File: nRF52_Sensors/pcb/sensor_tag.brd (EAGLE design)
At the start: 36.5 x 26.7 mm, 5 parts

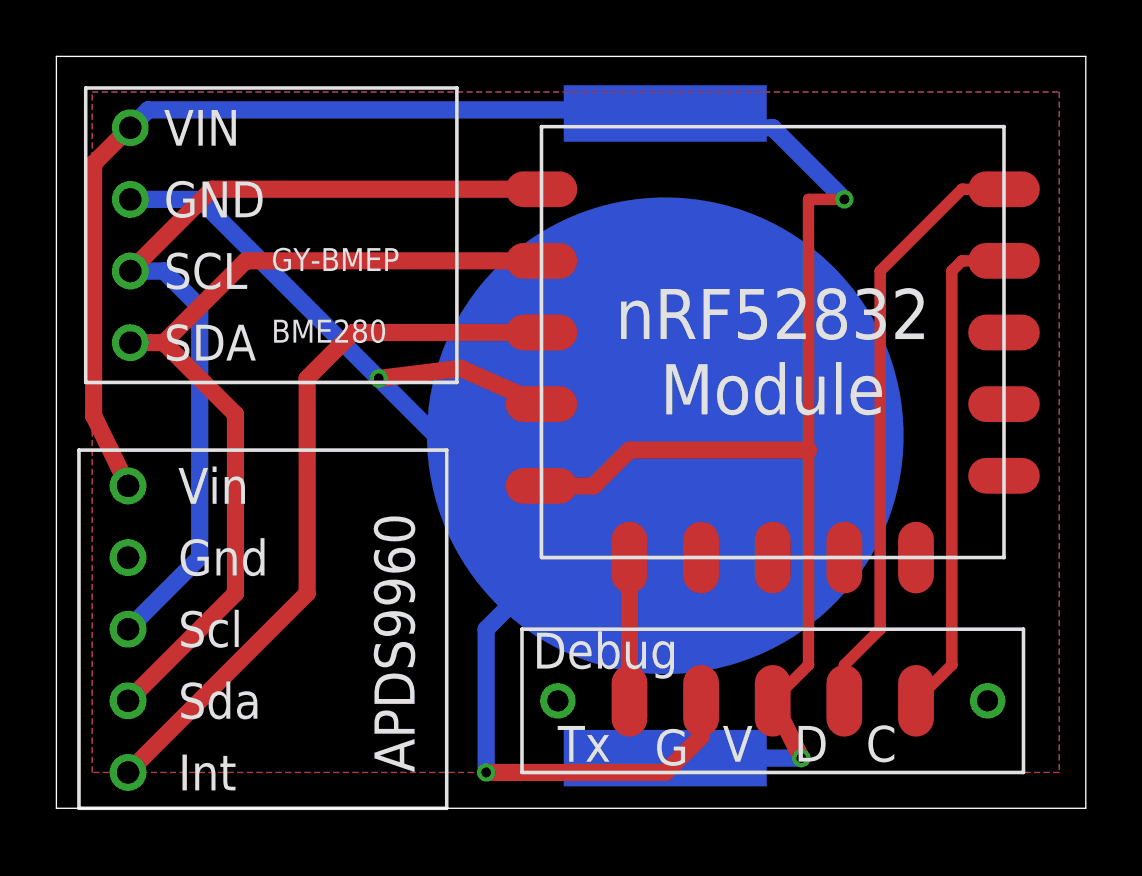
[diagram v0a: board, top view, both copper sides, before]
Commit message: nRF52 tests ongoing
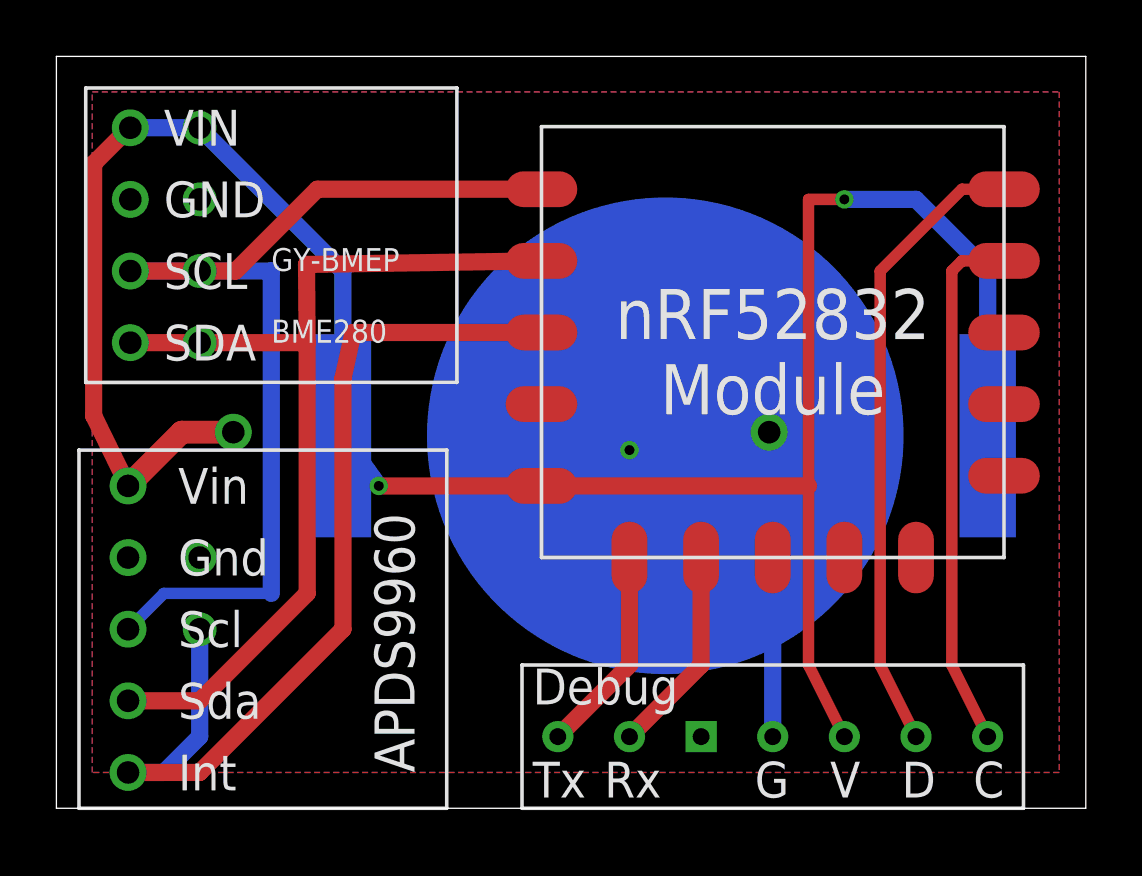
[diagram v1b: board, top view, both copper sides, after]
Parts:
- added U$6: CR2477, cr2477:CR2477
- moved U$5 1.27 mm to (25.4, 2.54)
- turned U$4 to 180 degrees
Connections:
- new net RX: U$3.P0_07, U$5.RX
- net GND: now also U$6.GND
- net SWCLK: now also U$5.SWDCLK; no longer U$5.SWCLK
- net VCC: now also U$6.VCC
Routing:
- net GND: track 51.8 -> 7.72 mm
- net INT: track 25.6 -> 33.8 mm, vias 0 -> 1
- net RX: track 0.00 -> 7.40 mm
- net SCL: track 31.2 -> 37.8 mm, vias 0 -> 1
- net VCC: track 77.1 -> 83.6 mm, vias 2 -> 3
- net SDA: track 31.2 -> 34.3 mm, vias 0 -> 1
- net TX: track 5.08 -> 7.40 mm
- net SWCLK: track 17.8 -> 18.8 mm
- net SWDIO: track 21.4 -> 22.4 mm
